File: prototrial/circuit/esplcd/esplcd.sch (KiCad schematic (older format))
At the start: 8 parts, among them U1 ESP-12E

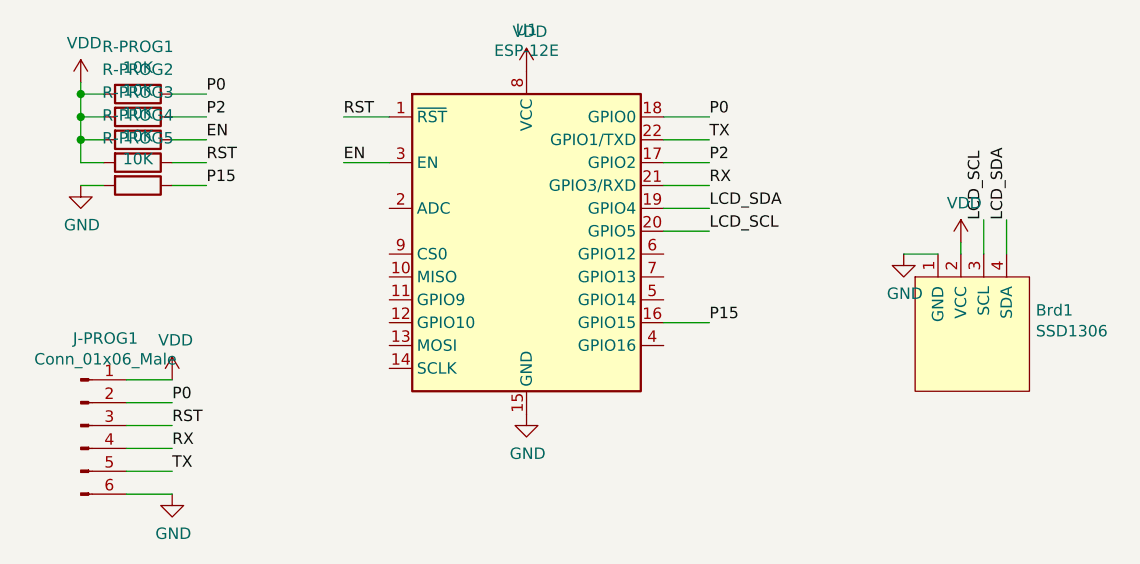
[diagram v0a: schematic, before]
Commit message: esp lcd draft
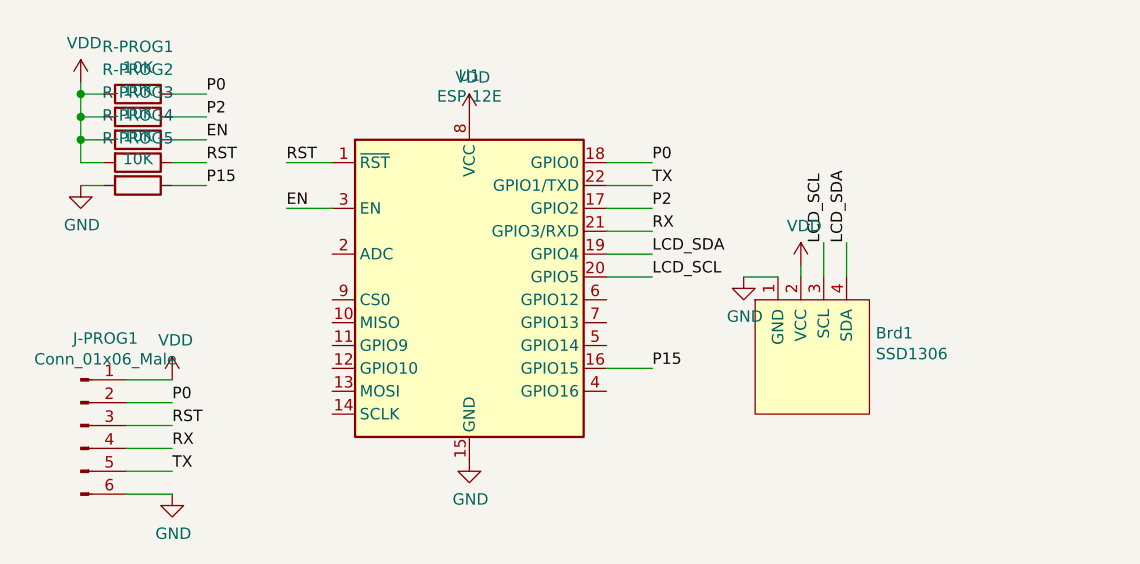
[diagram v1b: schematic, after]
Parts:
- J-PROG1: footprint (none) -> Connector_PinHeader_2.54mm:PinHeader_1x06_P2.54mm_Vertical
- R-PROG1, R-PROG2, R-PROG3, R-PROG4, R-PROG5: footprint (none) -> Resistor_SMD:R_0805_2012Metric_Pad1.20x1.40mm_HandSolder
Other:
- moved on the sheet: Brd1, U1
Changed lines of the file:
@@
 F 0 "J-PROG1" H 1608 3031 50  0000 C CNN
 F 1 "Conn_01x06_Male" H 1608 2940 50  0000 C CNN
-F 2 "" H 1500 2650 50  0001 C CNN
+F 2 "Connector_PinHeader_2.54mm:PinHeader_1x06_P2.54mm_Vertical" H 1500 2650 50  0001 C CNN
 F 3 "~" H 1500 2650 50  0001 C CNN
 	1    1500 2650
@@
 L power:GND #PWR06
 U 1 1 61EAA5F0
-P 3450 2600
-F 0 "#PWR06" H 3450 2350 50  0001 C CNN
-F 1 "GND" H 3455 2427 50  0000 C CNN
-F 2 "" H 3450 2600 50  0001 C CNN
-F 3 "" H 3450 2600 50  0001 C CNN
-	1    3450 2600
+P 3200 2800
+F 0 "#PWR06" H 3200 2550 50  0001 C CNN
+F 1 "GND" H 3205 2627 50  0000 C CNN
+F 2 "" H 3200 2800 50  0001 C CNN
+F 3 "" H 3200 2800 50  0001 C CNN
+	1    3200 2800
 	1    0    0    -1
 $EndComp
@@
 F 0 "R-PROG1" V 1543 1200 50  0000 C CNN
 F 1 "10K" V 1634 1200 50  0000 C CNN
-F 2 "" V 1680 1200 50  0001 C CNN
+F 2 "Resistor_SMD:R_0805_2012Metric_Pad1.20x1.40mm_HandSolder" V 1680 1200 50  0001 C CNN
 F 3 "~" H 1750 1200 50  0001 C CNN
 	1    1750 1200
@@
 F 0 "R-PROG2" V 1543 1300 50  0000 C CNN
 F 1 "10K" V 1634 1300 50  0000 C CNN
-F 2 "" V 1680 1300 50  0001 C CNN
+F 2 "Resistor_SMD:R_0805_2012Metric_Pad1.20x1.40mm_HandSolder" V 1680 1300 50  0001 C CNN
 F 3 "~" H 1750 1300 50  0001 C CNN
 	1    1750 1300
@@
 F 0 "R-PROG3" V 1543 1400 50  0000 C CNN
 F 1 "10K" V 1634 1400 50  0000 C CNN
-F 2 "" V 1680 1400 50  0001 C CNN
+F 2 "Resistor_SMD:R_0805_2012Metric_Pad1.20x1.40mm_HandSolder" V 1680 1400 50  0001 C CNN
 F 3 "~" H 1750 1400 50  0001 C CNN
 	1    1750 1400
@@
 F 0 "R-PROG4" V 1543 1500 50  0000 C CNN
 F 1 "10K" V 1634 1500 50  0000 C CNN
-F 2 "" V 1680 1500 50  0001 C CNN
+F 2 "Resistor_SMD:R_0805_2012Metric_Pad1.20x1.40mm_HandSolder" V 1680 1500 50  0001 C CNN
 F 3 "~" H 1750 1500 50  0001 C CNN
 	1    1750 1500
@@
 F 0 "R-PROG5" V 1543 1600 50  0000 C CNN
 F 1 "10K" V 1634 1600 50  0000 C CNN
-F 2 "" V 1680 1600 50  0001 C CNN
+F 2 "Resistor_SMD:R_0805_2012Metric_Pad1.20x1.40mm_HandSolder" V 1680 1600 50  0001 C CNN
 F 3 "~" H 1750 1600 50  0001 C CNN
 	1    1750 1600
@@
 L power:VDD #PWR05
 U 1 1 61EA8D9B
-P 3450 1100
-F 0 "#PWR05" H 3450 950 50  0001 C CNN
-F 1 "VDD" H 3465 1273 50  0000 C CNN
-F 2 "" H 3450 1100 50  0001 C CNN
-F 3 "" H 3450 1100 50  0001 C CNN
-	1    3450 1100
+P 3200 1300
+F 0 "#PWR05" H 3200 1150 50  0001 C CNN
+F 1 "VDD" H 3215 1473 50  0000 C CNN
+F 2 "" H 3200 1300 50  0001 C CNN
+F 3 "" H 3200 1300 50  0001 C CNN
+	1    3200 1300
 	1    0    0    -1
 $EndComp
@@
 L RF_Module:ESP-12E U1
 U 1 1 61EA2764
-P 3450 1900
-F 0 "U1" H 3450 2881 50  0000 C CNN
-F 1 "ESP-12E" H 3450 2790 50  0000 C CNN
-F 2 "RF_Module:ESP-12E" H 3450 1900 50  0001 C CNN
-F 3 "http://wiki.ai-thinker.com/_media/esp8266/esp8266_series_modules_user_manual_v1.1.pdf" H 3100 2000 50  0001 C CNN
-	1    3450 1900
-	1    0    0    -1
-$EndComp
-Text Label 4250 2200 0    50   ~ 0
+P 3200 2100
+F 0 "U1" H 3200 3081 50  0000 C CNN
+F 1 "ESP-12E" H 3200 2990 50  0000 C CNN
+F 2 "RF_Module:ESP-12E" H 3200 2100 50  0001 C CNN
+F 3 "http://wiki.ai-thinker.com/_media/esp8266/esp8266_series_modules_user_manual_v1.1.pdf" H 2850 2200 50  0001 C CNN
+	1    3200 2100
+	1    0    0    -1
+$EndComp
+Text Label 4000 2400 0    50   ~ 0
 P15
 Wire Wire Line
-	4050 2200 4250 2200
-Text Label 4250 1600 0    50   ~ 0
+	3800 2400 4000 2400
+Text Label 4000 1800 0    50   ~ 0
 RX
 Wire Wire Line
-	4050 1600 4250 1600
-Text Label 4250 1500 0    50   ~ 0
+	3800 1800 4000 1800
+Text Label 4000 1700 0    50   ~ 0
 P2
 Wire Wire Line
-	4050 1500 4250 1500
-Text Label 4250 1400 0    50   ~ 0
+	3800 1700 4000 1700
+Text Label 4000 1600 0    50   ~ 0
 TX
 Wire Wire Line
-	4050 1400 4250 1400
-Text Label 4250 1300 0    50   ~ 0
+	3800 1600 4000 1600
+Text Label 4000 1500 0    50   ~ 0
 P0
 Wire Wire Line
-	4050 1300 4250 1300
-Text Label 2650 1500 0    50   ~ 0
+	3800 1500 4000 1500
+Text Label 2400 1700 0    50   ~ 0
 EN
 Wire Wire Line
-	2850 1500 2650 1500
-Text Label 2650 1300 0    50   ~ 0
+	2600 1700 2400 1700
+Text Label 2400 1500 0    50   ~ 0
 RST
 Wire Wire Line
-	2850 1300 2650 1300
+	2600 1500 2400 1500
 Wire Wire Line
 	1900 1200 2050 1200
@@
 L SSD1306-128x64_OLED:SSD1306 Brd1
 U 1 1 61EA6811
-P 5400 2250
-F 0 "Brd1" H 5678 2354 50  0000 L CNN
-F 1 "SSD1306" H 5678 2263 50  0000 L CNN
-F 2 "SSD1306:128x64OLED" H 5400 2500 50  0001 C CNN
-F 3 "" H 5400 2500 50  0001 C CNN
-	1    5400 2250
-	1    0    0    -1
-$EndComp
-Wire Wire Line
-	4050 1700 4250 1700
-Wire Wire Line
-	4050 1800 4250 1800
-Text Label 4250 1700 0    50   ~ 0
+P 4700 2350
+F 0 "Brd1" H 4978 2454 50  0000 L CNN
+F 1 "SSD1306" H 4978 2363 50  0000 L CNN
+F 2 "SSD1306:128x64OLED" H 4700 2600 50  0001 C CNN
+F 3 "" H 4700 2600 50  0001 C CNN
+	1    4700 2350
+	1    0    0    -1
+$EndComp
+Wire Wire Line
+	3800 1900 4000 1900
+Wire Wire Line
+	3800 2000 4000 2000
+Text Label 4000 1900 0    50   ~ 0
 LCD_SDA
-Text Label 4250 1800 0    50   ~ 0
+Text Label 4000 2000 0    50   ~ 0
 LCD_SCL
 $Comp
 L power:VDD #PWR08
 U 1 1 61EA9A75
-P 5350 1850
-F 0 "#PWR08" H 5350 1700 50  0001 C CNN
-F 1 "VDD" H 5365 2023 50  0000 C CNN
-F 2 "" H 5350 1850 50  0001 C CNN
-F 3 "" H 5350 1850 50  0001 C CNN
-	1    5350 1850
+P 4650 1950
+F 0 "#PWR08" H 4650 1800 50  0001 C CNN
+F 1 "VDD" H 4665 2123 50  0000 C CNN
+F 2 "" H 4650 1950 50  0001 C CNN
+F 3 "" H 4650 1950 50  0001 C CNN
+	1    4650 1950
 	1    0    0    -1
 $EndComp
@@
 L power:GND #PWR07
 U 1 1 61EAA146
-P 5100 1900
-F 0 "#PWR07" H 5100 1650 50  0001 C CNN
-F 1 "GND" H 5105 1727 50  0000 C CNN
-F 2 "" H 5100 1900 50  0001 C CNN
-F 3 "" H 5100 1900 50  0001 C CNN
-	1    5100 1900
-	1    0    0    -1
-$EndComp
-Wire Wire Line
-	5350 1850 5350 1900
-Wire Wire Line
-	5250 1900 5100 1900
-Text Label 5450 1750 1    50   ~ 0
+P 4400 2000
+F 0 "#PWR07" H 4400 1750 50  0001 C CNN
+F 1 "GND" H 4405 1827 50  0000 C CNN
+F 2 "" H 4400 2000 50  0001 C CNN
+F 3 "" H 4400 2000 50  0001 C CNN
+	1    4400 2000
+	1    0    0    -1
+$EndComp
+Wire Wire Line
+	4650 1950 4650 2000
+Wire Wire Line
+	4550 2000 4400 2000
+Text Label 4750 1850 1    50   ~ 0
 LCD_SCL
-Text Label 5550 1750 1    50   ~ 0
+Text Label 4850 1850 1    50   ~ 0
 LCD_SDA
 Wire Wire Line
-	5450 1900 5450 1750
-Wire Wire Line
-	5550 1900 5550 1750
+	4750 2000 4750 1850
+Wire Wire Line
+	4850 2000 4850 1850
 $EndSCHEMATC
